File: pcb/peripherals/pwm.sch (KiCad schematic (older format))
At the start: 24 parts, among them J5 JST XH, J6 JST XH, J7 JST XH, J8 JST XH, Q1 FDD8447L, Q2 FDD8447L, Q3 FDD8447L, Q4 FDD8447L

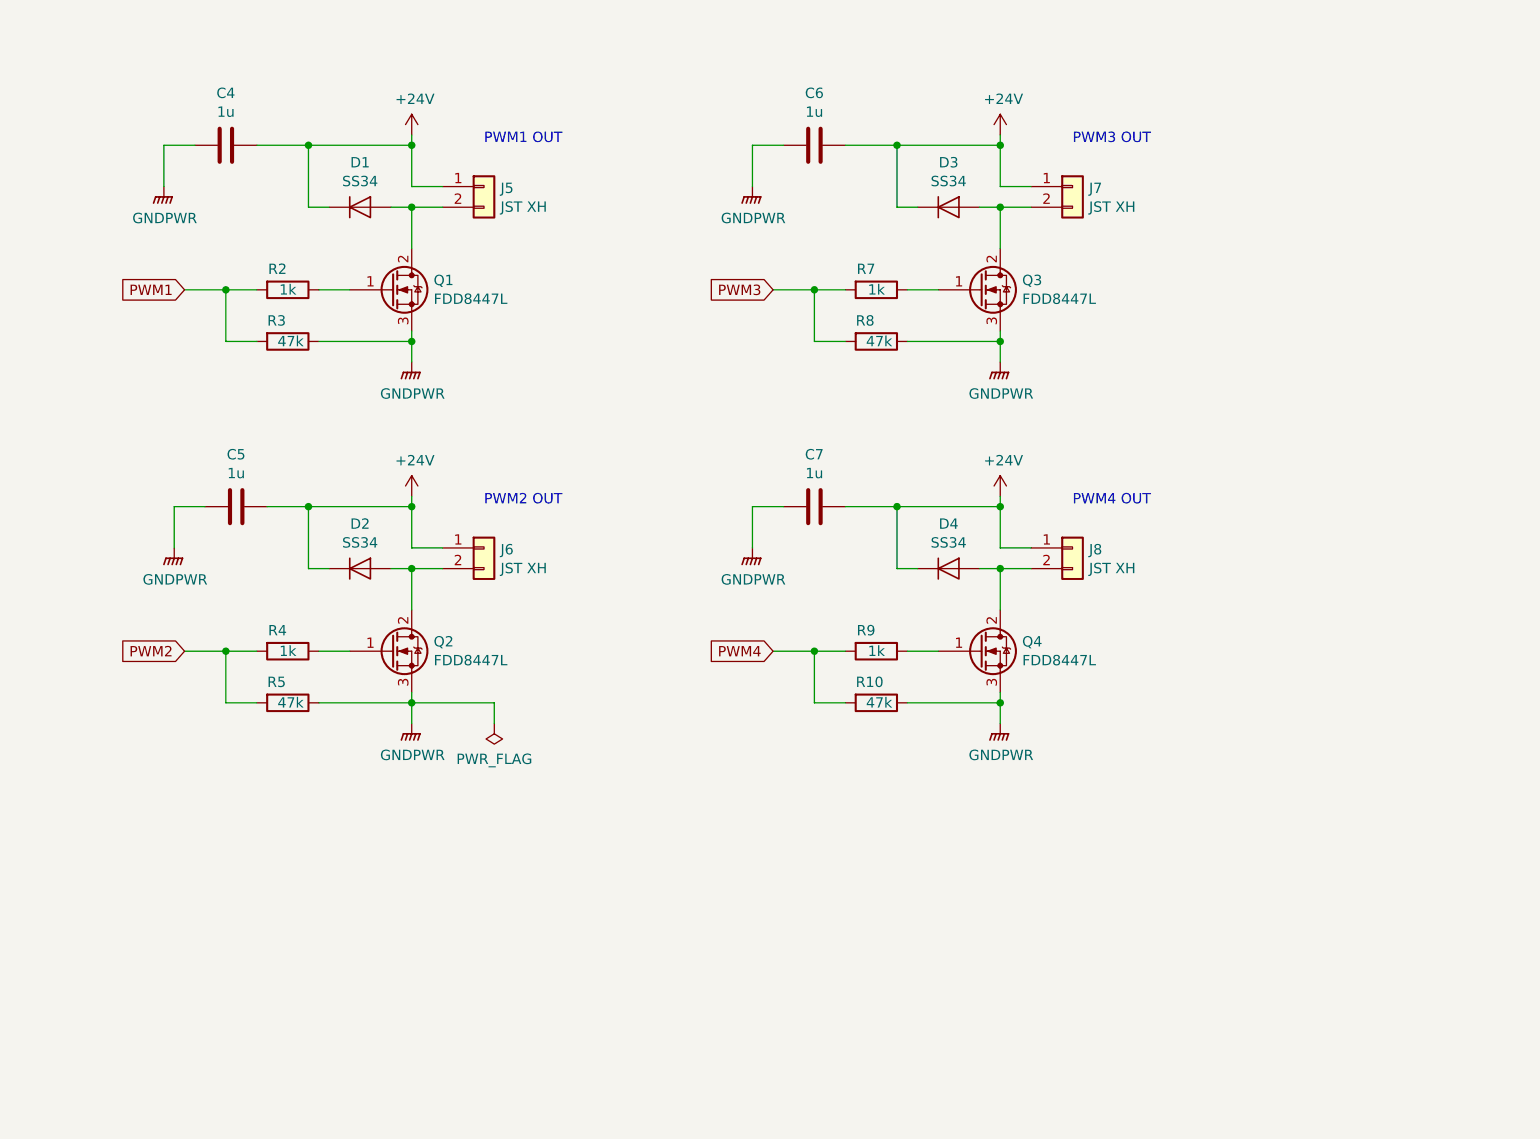
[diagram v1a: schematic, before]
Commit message: Work on layout.
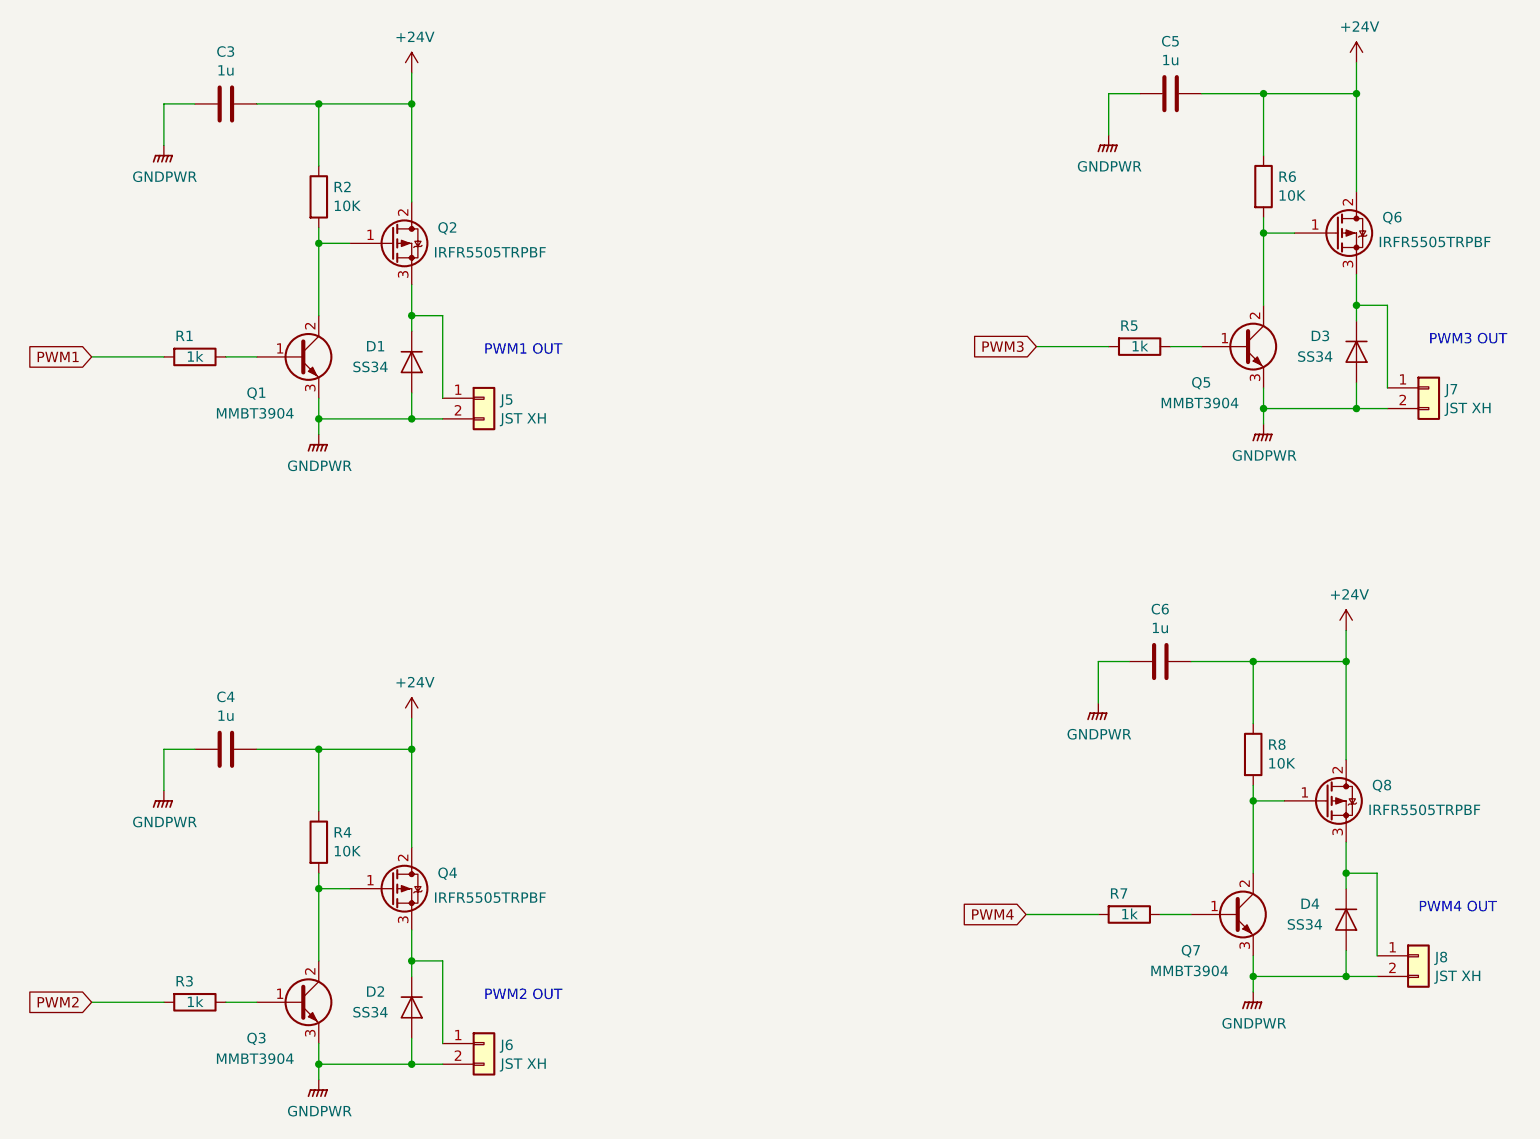
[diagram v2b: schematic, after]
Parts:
- removed C7: 1u, Capacitor_SMD:C_0805_2012Metric, symbol Device:C
- removed Q1, Q2, Q3, Q4: FDD8447L, Package_TO_SOT_SMD:TO-252-2, symbol Device:Q_NMOS_GDS
- removed R10: 47k, Resistor_SMD:R_0603_1608Metric, symbol Device:R
- removed R9: 1k, Resistor_SMD:R_0603_1608Metric, symbol Device:R
- added C4: 1u, Capacitor_SMD:C_0805_2012Metric, symbol Device:C
- added Q1, Q3, Q5, Q7: MMBT3904, Package_TO_SOT_SMD:SOT-23, symbol Device:Q_NPN_BCE
- added Q2, Q4, Q6, Q8: IRFR5505TRPBF, Package_TO_SOT_SMD:TO-252-3_TabPin2, symbol Device:Q_PMOS_GDS
- added R2, R6: 10K, Resistor_SMD:R_0603_1608Metric, symbol Device:R
- R3, R5: value 47k -> 1k
- R4: value 1k -> 10K
- R8: value 47k -> 10K
- renumbered C4 to C3, R2 to R1
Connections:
- net +24V: now also R4.1, R8.1, C4.1, Q2.2 (D), Q4.2 (D), Q6.2 (D), Q8.2 (D), R2.1, R6.1; no longer D1.1 (K), D2.1 (K), D3.1 (K), D4.1 (K), J5.1 (Pin_1), J6.1 (Pin_1), J7.1 (Pin_1), J8.1 (Pin_1)
- net GNDPWR: now also D1.2 (A), D2.2 (A), D3.2 (A), D4.2 (A), J5.2 (Pin_2), J6.2 (Pin_2), J7.2 (Pin_2), J8.2 (Pin_2), C4.2, Q1.3 (E), Q3.3 (E), Q5.3 (E), Q7.3 (E); no longer R3.1, R5.1, R8.1
- net PWM1: no longer R3.2
- net PWM2: now also R3.2; no longer R4.2, R5.2
- net PWM3: now also R5.2; no longer R7.2, R8.2
- net PWM4: now also R7.2
- net at R1.1: now also Q1.1 (B)
- net at R7.1: now also Q7.1 (B)
- new net: D1.1 (K), J5.1 (Pin_1), Q2.3 (S)
- new net: Q1.2 (C), Q2.1 (G), R2.2
- new net: D2.1 (K), J6.1 (Pin_1), Q4.3 (S)
- new net: Q3.1 (B), R3.1
- new net: Q3.2 (C), Q4.1 (G), R4.2
- new net: D3.1 (K), J7.1 (Pin_1), Q6.3 (S)
- new net: Q5.1 (B), R5.1
- new net: Q5.2 (C), Q6.1 (G), R6.2
- new net: D4.1 (K), J8.1 (Pin_1), Q8.3 (S)
- new net: Q7.2 (C), Q8.1 (G), R8.2
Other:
- moved on the sheet: C3, D1, J5, R1
